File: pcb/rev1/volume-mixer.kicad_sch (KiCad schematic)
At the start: 121 parts, among them CON1 TC2030-IDC, J1 Conn_01x04_Pin, J10 Conn_01x04_Pin, J2 Conn_01x10_Pin, J3 Conn_01x10_Pin, J4 Conn_01x04_Pin, J5 JST, J6 Conn_01x04_Pin, J7 Conn_01x04_Pin, J8 Conn_01x04_Pin, J9 Conn_01x04_Pin, Q1 NMOS, Q10 NMOS, Q3 NMOS, Q7 NMOS, Q8 NMOS, Q9 NMOS, SW1 SW_Push, SW2 SW_Push, SW3 SW_Push, U1 STM32F302C8Tx, U2 24LC64, U3 XC6206PxxxMR, U4 XC6206PxxxMR, U5 PRTR5V0U2X, U6 TCA9548APWR, Y1 8MHz

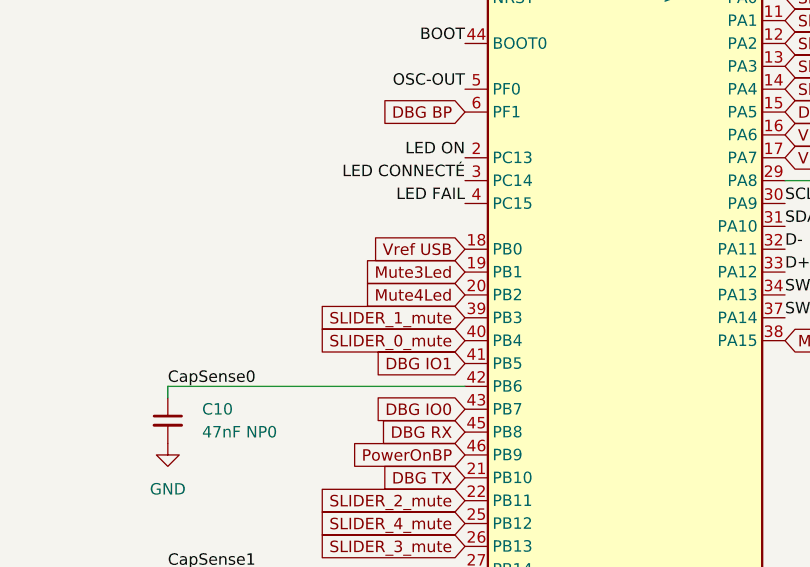
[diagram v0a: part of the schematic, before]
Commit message: BIDIBOU
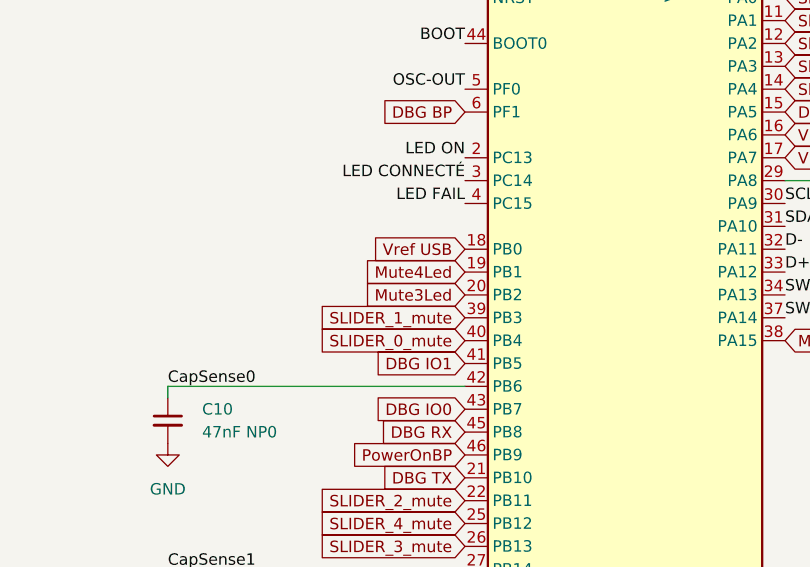
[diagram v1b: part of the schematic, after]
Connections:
- net Mute3Led: now also U1.20 (PB2); no longer U1.19 (PB1)
- net Mute4Led: now also U1.19 (PB1); no longer U1.20 (PB2)
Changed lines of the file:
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@@
 	(global_label "Mute3Led"
 		(shape input)
+		(at 67.31 81.28 180)
+		(fields_autoplaced yes)
+		(effects
+			(font
+				(size 1.27 1.27)
+			)
+			(justify right)
+		)
+		(property "Intersheetrefs" "${INTERSHEET_REFS}"
+			(at 55.4349 81.28 0)
+			(effects
+				(font
+					(size 1.27 1.27)
+				)
+				(justify right)
+				(hide yes)
+			)
+		)
+	)
+	(global_label "DBG RX"
+		(shape input)
+		(at 213.36 105.41 0)
+		(fields_autoplaced yes)
+		(effects
+			(font
+				(size 1.27 1.27)
+			)
+			(justify left)
+		)
+		(property "Intersheetrefs" "${INTERSHEET_REFS}"
+			(at 223.6023 105.41 0)
+			(effects
+				(font
+					(size 1.27 1.27)
+				)
+				(justify left)
+				(hide yes)
+			)
+		)
+	)
+	(global_label "Mute4Led"
+		(shape input)
 		(at 67.31 78.74 180)
 		(fields_autoplaced yes)
@@
 		)
 	)
-	(global_label "DBG RX"
-		(shape input)
-		(at 213.36 105.41 0)
-		(fields_autoplaced yes)
-		(effects
-			(font
-				(size 1.27 1.27)
-			)
-			(justify left)
-		)
-		(property "Intersheetrefs" "${INTERSHEET_REFS}"
-			(at 223.6023 105.41 0)
-			(effects
-				(font
-					(size 1.27 1.27)
-				)
-				(justify left)
+	(global_label "Mute2Led"
+		(shape input)
+		(at 67.31 114.3 180)
+		(fields_autoplaced yes)
+		(effects
+			(font
+				(size 1.27 1.27)
+			)
+			(justify right)
+		)
+		(property "Intersheetrefs" "${INTERSHEET_REFS}"
+			(at 55.4349 114.3 0)
+			(effects
+				(font
+					(size 1.27 1.27)
+				)
+				(justify right)
 				(hide yes)
 			)
@@
 	(global_label "Mute4Led"
 		(shape input)
-		(at 67.31 81.28 180)
-		(fields_autoplaced yes)
-		(effects
-			(font
-				(size 1.27 1.27)
-			)
-			(justify right)
-		)
-		(property "Intersheetrefs" "${INTERSHEET_REFS}"
-			(at 55.4349 81.28 0)
-			(effects
-				(font
-					(size 1.27 1.27)
-				)
-				(justify right)
-				(hide yes)
-			)
-		)
-	)
-	(global_label "Mute2Led"
-		(shape input)
-		(at 67.31 114.3 180)
-		(fields_autoplaced yes)
-		(effects
-			(font
-				(size 1.27 1.27)
-			)
-			(justify right)
-		)
-		(property "Intersheetrefs" "${INTERSHEET_REFS}"
-			(at 55.4349 114.3 0)
-			(effects
-				(font
-					(size 1.27 1.27)
-				)
-				(justify right)
-				(hide yes)
-			)
-		)
-	)
-	(global_label "Mute4Led"
-		(shape input)
 		(at 328.93 55.88 90)
 		(fields_autoplaced yes)
@@
 			)
 		)
-	)
-	(rule_area
-		(polyline
-			(pts
-				(xy 271.78 153.67) (xy 297.18 153.67) (xy 297.18 181.61) (xy 271.78 181.61)
-			)
-			(stroke
-				(width 0)
-				(type dash)
-			)
-			(fill
-				(type none)
-			)
-		)
-	)
-	(netclass_flag ""
-		(length 2.54)
-		(shape round)
-		(at 271.78 158.75 90)
-		(fields_autoplaced yes)
-		(effects
-			(font
-				(size 1.27 1.27)
-			)
-			(justify left bottom)
-		)
-		(property "Netclass" "Net_Isolé"
-			(at 269.24 158.0515 90)
-			(effects
-				(font
-					(size 1.27 1.27)
-				)
-				(justify left)
-			)
-		)
-		(property "Component Class" ""
-			(at -148.59 2.54 0)
-			(effects
-				(font
-					(size 1.27 1.27)
-					(italic yes)
-				)
-			)
-		)

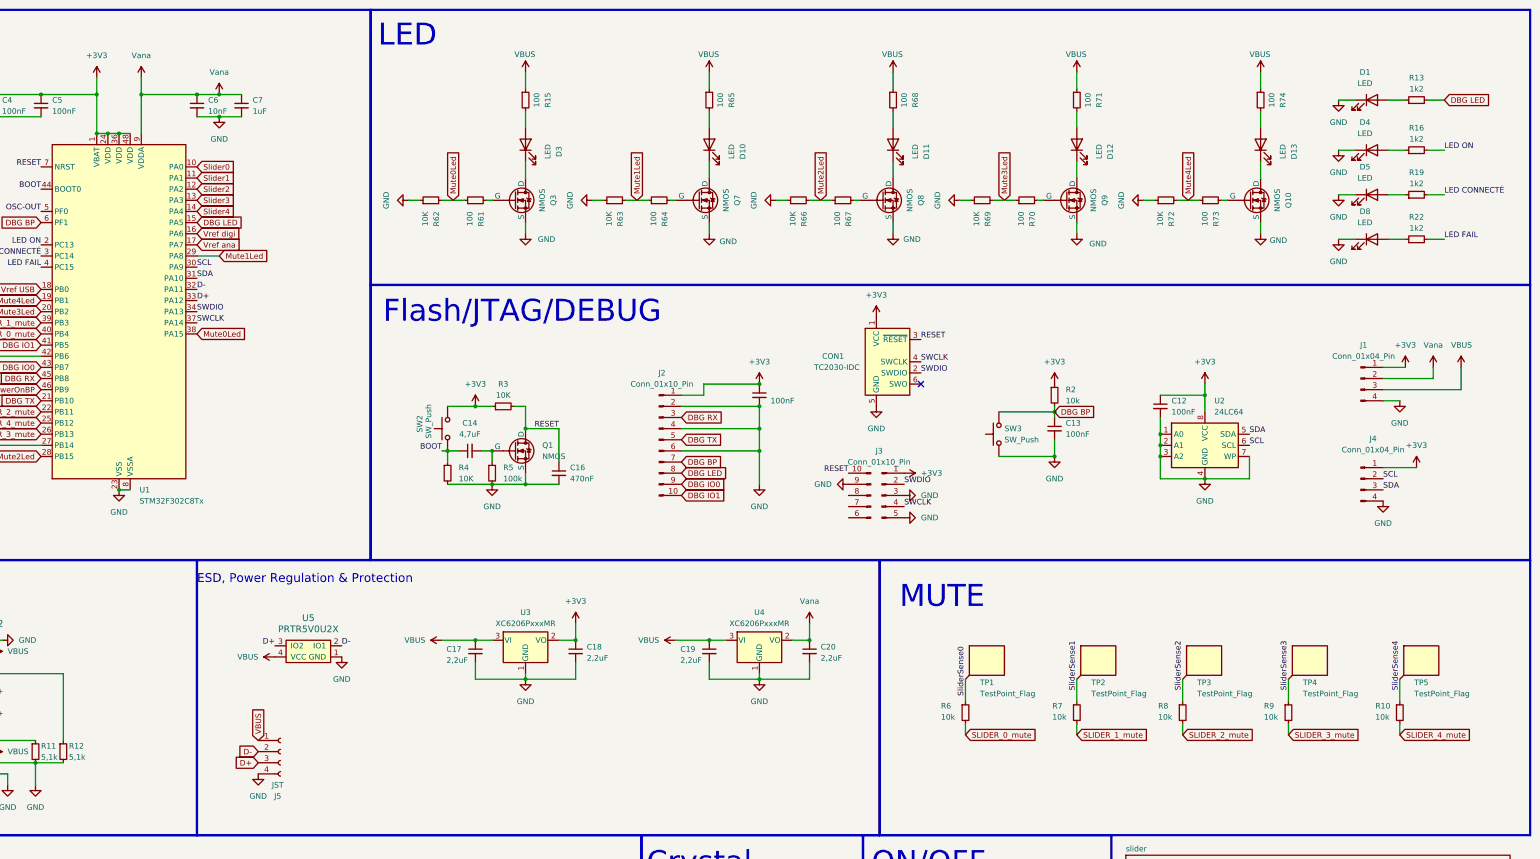
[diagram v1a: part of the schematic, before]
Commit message: BIDIBOU
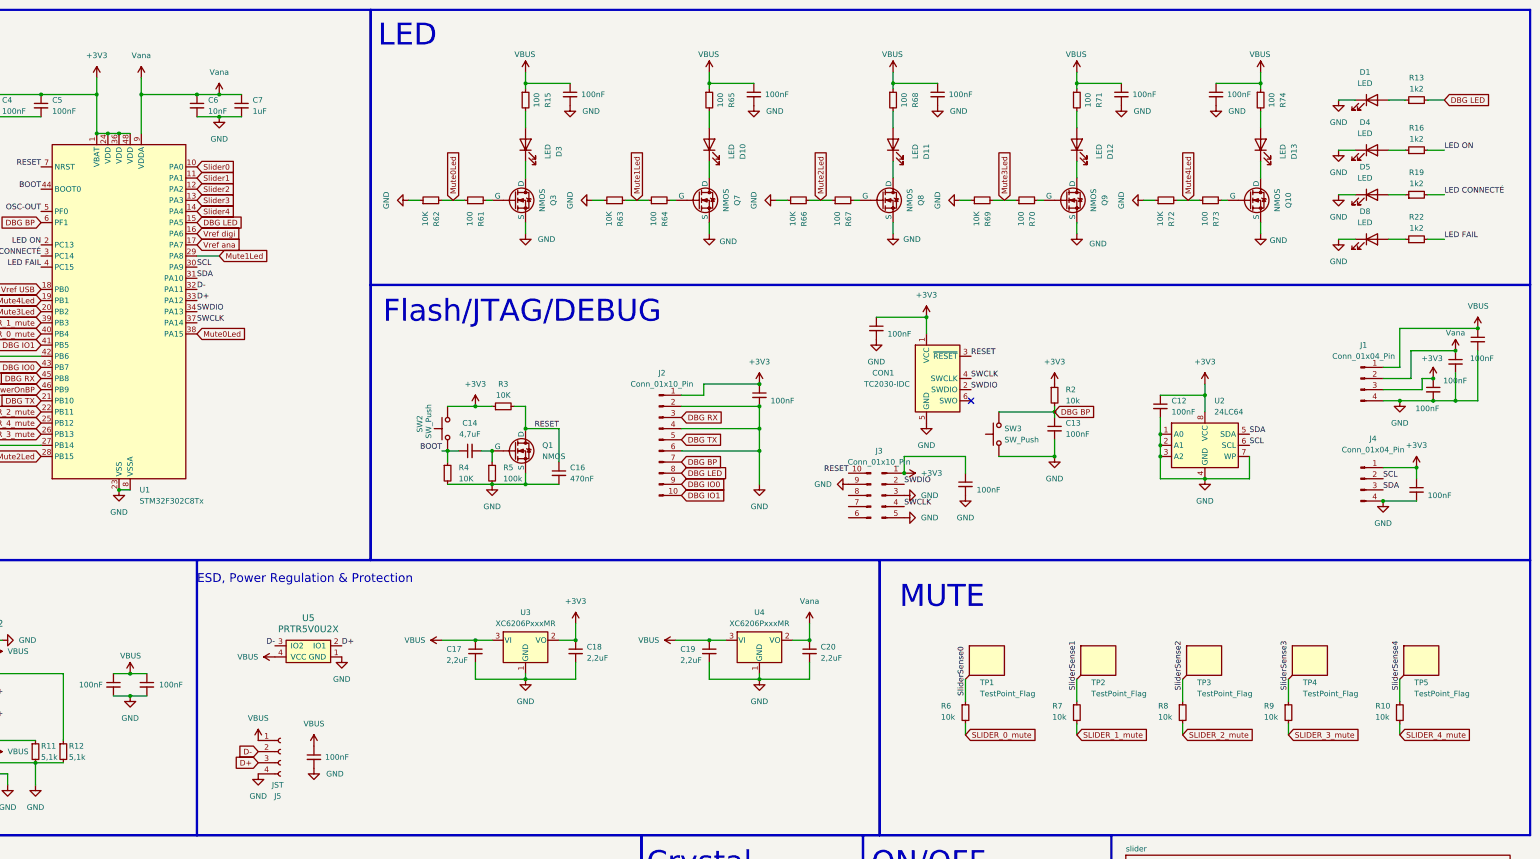
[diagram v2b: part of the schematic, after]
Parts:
- added C43, C44, C45, C46, C47, C48, C49, C50, C51, C52, C53, C54, C55, C56: 100nF, Capacitor_SMD:C_0603_1608Metric, symbol Device:C_Small
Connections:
- net +3V3: now also J1.3 (Pin_3), C43.1, C44.1, C45.1, C46.1; no longer J1.1 (Pin_1)
- net D+: now also U5.2 (IO1); no longer U5.3 (IO2)
- net D-: now also U5.3 (IO2); no longer U5.2 (IO1)
- net GND: now also C43.2, C44.2, C45.2, C46.2, C47.2, C48.2, C49.2, C50.2, C51.2, C52.2, C53.2, C54.2, C55.2, C56.2
- net VBUS: now also J1.1 (Pin_1), C48.1, C49.1, C50.1, C51.1, C52.1, C53.1, C54.1, C55.1, C56.1; no longer J1.3 (Pin_3)
- net Vana: now also C47.1
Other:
- moved on the sheet: CON1
